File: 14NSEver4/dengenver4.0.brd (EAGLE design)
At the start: 80 x 25.4 mm, 44 parts, among them Q1 16mhz, SW2 SRIDE_SWITCH

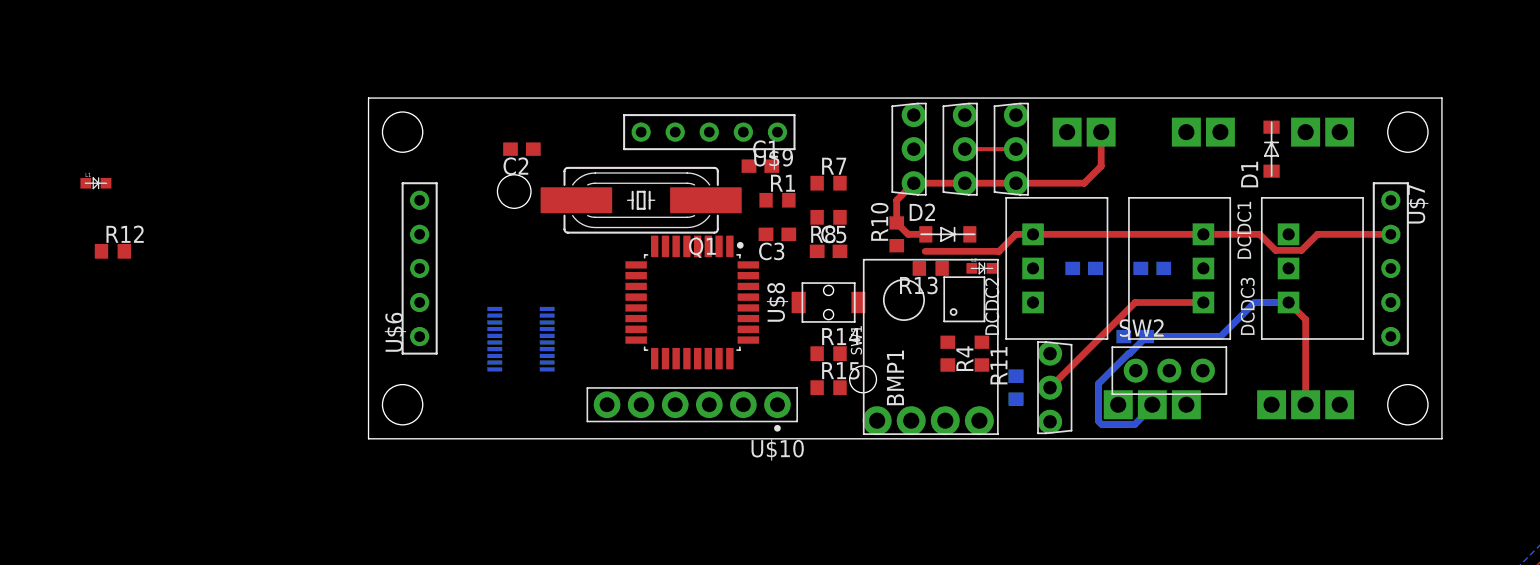
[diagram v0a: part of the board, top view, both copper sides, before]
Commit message: Completed board files ver1.0
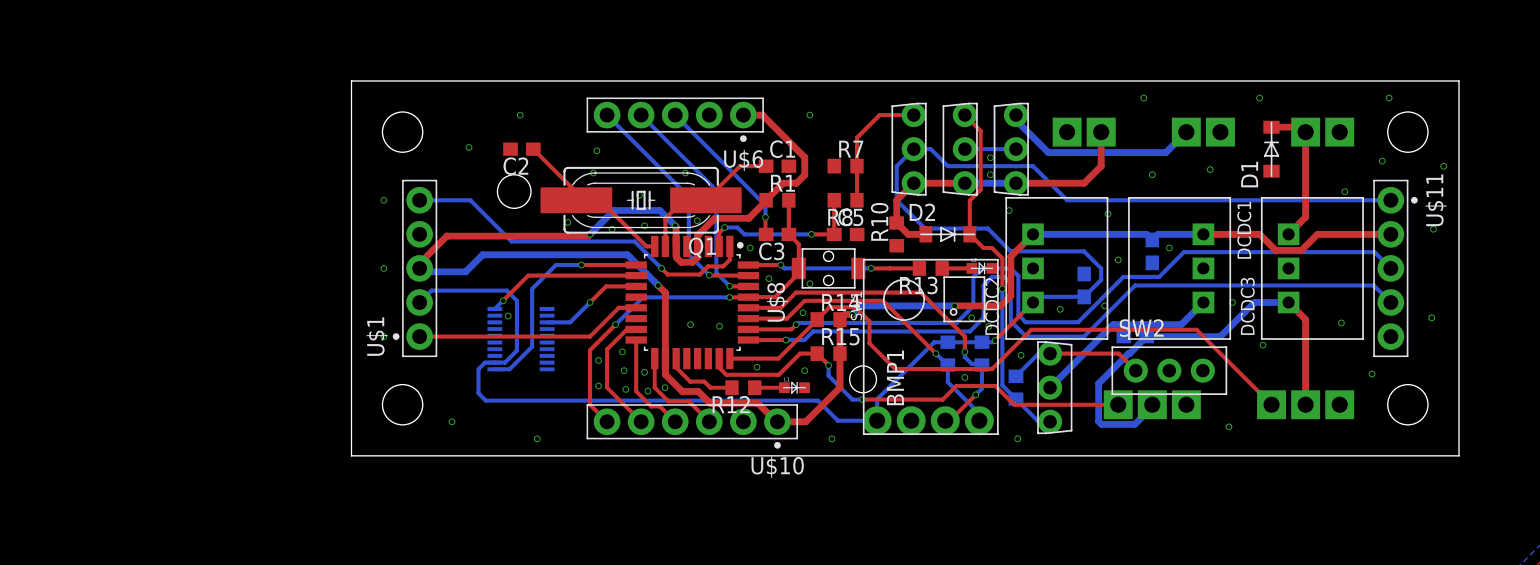
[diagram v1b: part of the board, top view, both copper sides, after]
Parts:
- removed U$7, U$9: 1X5, PinSocket:1X5
- added U$1, U$11: 1X5, pin_socket:HDRVR5W64P254_1X5_1310X250X865B
- U$6: device PinSocket:1X5 -> pin_socket:HDRVR5W64P254_1X5_1310X250X865B
- moved L1 54.3 mm to (31.8, 3.81)
- moved R12 48.1 mm to (27.9, 3.81), turned to 180 degrees
- moved U$6 29.2 mm to (27.9, 24.1), turned to 180 degrees
- moved R14 2.54 mm to (34.3, 8.89)
- moved R15 2.54 mm to (34.3, 6.35)
- moved SW1 2.54 mm to (34.3, 12.7)
- moved C5 1.80 mm to (35.6, 15.2)
- moved R7 1.80 mm to (35.6, 20.3)
- moved R8 1.80 mm to (35.6, 17.8)
- moved C4 1.27 mm to (58.4, 14.0), turned to 270 degrees
- moved U$10 1.27 mm to (30.5, 1.27)
- moved C1 1.27 mm to (30.5, 20.3)
- moved C6 1.27 mm to (53.3, 11.4), turned to 90 degrees
- flipped R11 to the bottom, turned to 90 degrees
- flipped R4 to the bottom, turned to 90 degrees
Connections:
- net +3V3: now also U$1.2, U$11.1; no longer U$6.P$2, U$7.P$1
- net +5V: now also U$1.3, U$11.2, U$6.1; no longer U$6.P$3, U$7.P$2, U$9.P$1
- net BORD1: now also U$1.5; no longer U$6.P$5
- net BORD2: now also U$1.1; no longer U$6.P$1
- net BORDRX: now also U$11.3; no longer U$7.P$3
- net BORDTX: now also U$11.4; no longer U$7.P$4
- net GND: now also U$1.4, U$11.5, U$6.2; no longer U$6.P$4, U$7.P$5, U$9.P$2
- net LED_1.1: now also U$8.ADC6
- net RESET: now also U$6.3; no longer U$9.P$3
- net RX: now also U$6.4; no longer U$9.P$4
- net TX: now also U$6.5; no longer U$9.P$5
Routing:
- net +3V3: track 0.00 -> 129.2 mm, vias 0 -> 1
- net +5V: track 36.2 -> 138.1 mm, vias 0 -> 5
- net BORDRX: track 0.00 -> 57.1 mm, vias 0 -> 1
- net BORDTX: track 0.00 -> 56.8 mm, vias 0 -> 1
- net SERVO1: track 0.00 -> 48.4 mm
- net SERVO2: track 0.00 -> 34.2 mm, vias 0 -> 2
- net RESETB: track 0.00 -> 29.5 mm, vias 0 -> 2
- net N$3: track 0.00 -> 27.0 mm, vias 0 -> 1
- net BORD1: track 0.00 -> 26.9 mm, vias 0 -> 1
- net SCL: track 0.00 -> 26.5 mm, vias 0 -> 2
- net SDA: track 0.00 -> 22.5 mm, vias 0 -> 1
- net TX: track 0.00 -> 18.0 mm, vias 0 -> 1
- net BORD2: track 0.00 -> 17.0 mm
- net RX: track 0.00 -> 16.9 mm, vias 0 -> 1
- net IM_RESET: track 0.00 -> 16.3 mm, vias 0 -> 1
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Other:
- board size 80 x 25.4 mm -> 82.5 x 27.9 mm
